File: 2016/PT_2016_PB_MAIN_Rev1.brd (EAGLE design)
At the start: 150.9 x 201.9 mm, 137 parts, among them M1+ ANDERSON_POWERPOLEPP45_PCB_HO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, M1- ANDERSON_POWERPOLEPP45_PCB_HO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, M2+ ANDERSON_POWERPOLEPP45_PCB_HO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, M2- ANDERSON_POWERPOLEPP45_PCB_HO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, M3+ ANDERSON_POWERPOLEPP45_PCB_HO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, M3- ANDERSON_POWERPOLEPP45_PCB_HO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, M4+ ANDERSON_POWERPOLEPP45_PCB_HO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, M4- ANDERSON_POWERPOLEPP45_PCB_HO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, M5+ ANDERSON_POWERPOLEPP45_PCB_HO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, M5- ANDERSON_POWERPOLEPP45_PCB_HO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, M6+ ANDERSON_POWERPOLEPP45_PCB_HO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, M6- ANDERSON_POWERPOLEPP45_PCB_HO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, Q1 Q_IRFS7437PbF, Q11 Q_IRFS7437PbF, Q12 2N7002, Q14 Q_IRFS7437PbF, Q16 Q_IRFS7437PbF, Q2 2N7002, Q20 Q_IRFS7437PbF, Q6 Q_IRFS7437PbF, Q7 Q_IRFS7437PbF, Q9 Q_IRFS7437PbF

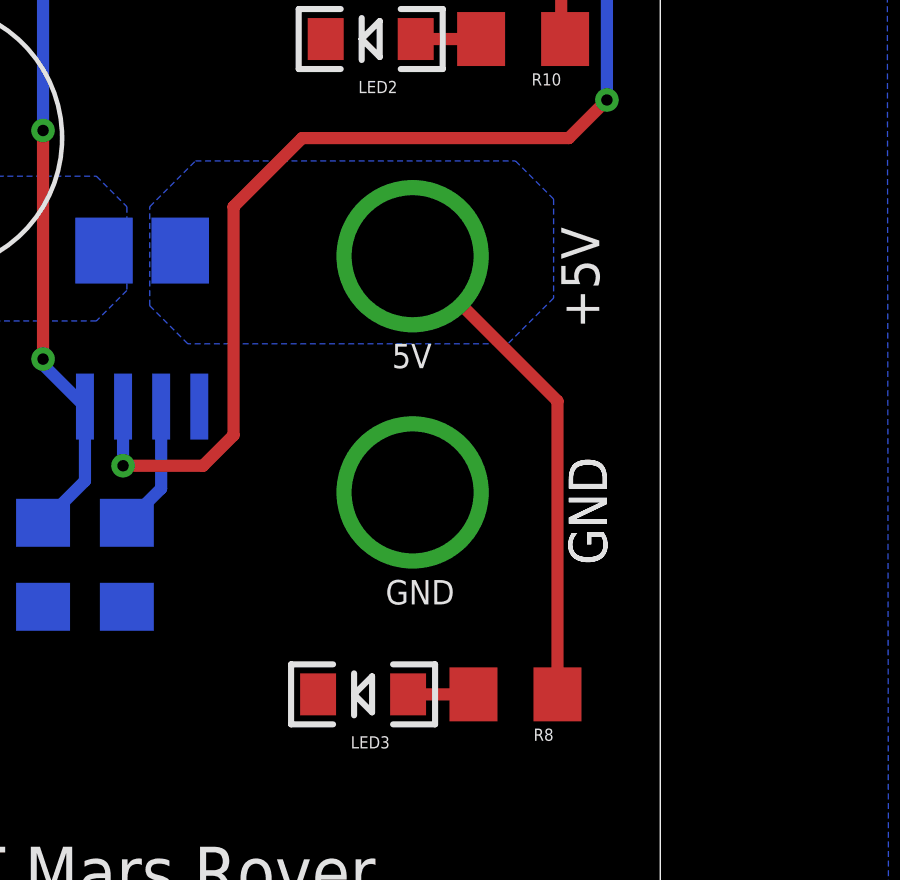
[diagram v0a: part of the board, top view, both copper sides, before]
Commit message: gen gerbers for rev 1
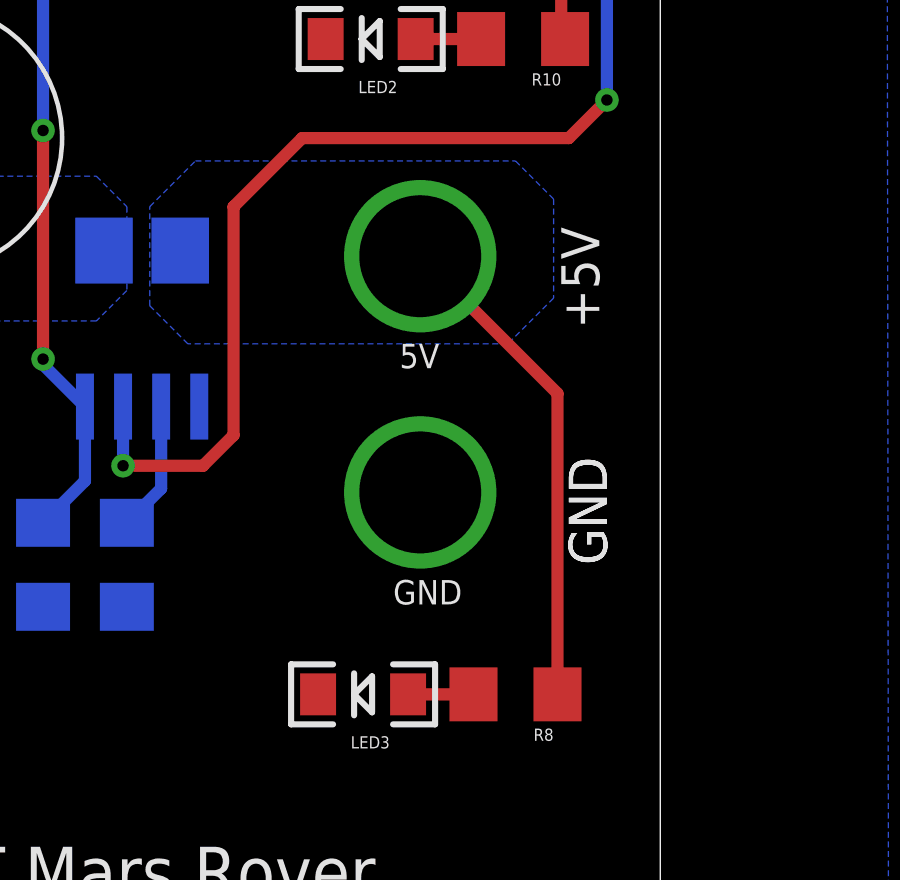
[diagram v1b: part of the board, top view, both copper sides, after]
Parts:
- moved U$45 0.25 mm to (134.1, 14.2)
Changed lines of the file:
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@@
 <layer number="16" name="Bottom" color="1" fill="1" visible="yes" active="yes"/>
 <layer number="17" name="Pads" color="2" fill="1" visible="yes" active="yes"/>
-<layer number="18" name="Vias" color="2" fill="1" visible="no" active="yes"/>
-<layer number="19" name="Unrouted" color="6" fill="1" visible="no" active="yes"/>
-<layer number="20" name="Dimension" color="15" fill="1" visible="no" active="yes"/>
+<layer number="18" name="Vias" color="2" fill="1" visible="yes" active="yes"/>
+<layer number="19" name="Unrouted" color="6" fill="1" visible="yes" active="yes"/>
+<layer number="20" name="Dimension" color="15" fill="1" visible="yes" active="yes"/>
 <layer number="21" name="tPlace" color="7" fill="1" visible="yes" active="yes"/>
-<layer number="22" name="bPlace" color="7" fill="1" visible="no" active="yes"/>
-<layer number="23" name="tOrigins" color="15" fill="1" visible="no" active="yes"/>
-<layer number="24" name="bOrigins" color="15" fill="1" visible="no" active="yes"/>
+<layer number="22" name="bPlace" color="7" fill="1" visible="yes" active="yes"/>
+<layer number="23" name="tOrigins" color="15" fill="1" visible="yes" active="yes"/>
+<layer number="24" name="bOrigins" color="15" fill="1" visible="yes" active="yes"/>
 <layer number="25" name="tNames" color="7" fill="1" visible="no" active="yes"/>
 <layer number="26" name="bNames" color="7" fill="1" visible="no" active="yes"/>
@@
 <layer number="47" name="Measures" color="7" fill="1" visible="no" active="yes"/>
 <layer number="48" name="Document" color="7" fill="1" visible="no" active="yes"/>
-<layer number="49" name="Reference" color="7" fill="1" visible="yes" active="yes"/>
+<layer number="49" name="Reference" color="7" fill="1" visible="no" active="yes"/>
 <layer number="50" name="dxf" color="7" fill="1" visible="no" active="yes"/>
-<layer number="51" name="tDocu" color="7" fill="1" visible="no" active="yes"/>
-<layer number="52" name="bDocu" color="7" fill="1" visible="no" active="yes"/>
+<layer number="51" name="tDocu" color="7" fill="1" visible="yes" active="yes"/>
+<layer number="52" name="bDocu" color="7" fill="1" visible="yes" active="yes"/>
 <layer number="91" name="Nets" color="2" fill="1" visible="no" active="no"/>
 <layer number="92" name="Busses" color="1" fill="1" visible="no" active="no"/>
@@
 <attribute name="COLOR1" value="" x="-16.256" y="4.572" size="1.778" layer="27" display="off"/>
 </element>
-<element name="U$45" library="MRDT-Connectors" package="APP_5V_VERT_CONFIG" value="APP_2POS_CONFIG5V_VERT" x="133.858" y="14.224">
-<attribute name="COLOR2" value="BLACK" x="133.858" y="14.224" size="1.778" layer="27" display="off"/>
-<attribute name="COLOR1" value="RED" x="133.858" y="14.224" size="1.778" layer="27" display="off"/>
+<element name="U$45" library="MRDT-Connectors" package="APP_5V_VERT_CONFIG" value="APP_2POS_CONFIG5V_VERT" x="134.112" y="14.224">
+<attribute name="COLOR2" value="BLACK" x="134.112" y="14.224" size="1.778" layer="27" display="off"/>
+<attribute name="COLOR1" value="RED" x="134.112" y="14.224" size="1.778" layer="27" display="off"/>
 </element>
 <element name="U$46" library="MRDT-Connectors" package="APP_12V_VERT_CONFIG" value="APP_2POS_CONFIG12V_VERT" x="134.112" y="36.068">
@@
 </polygon>
 <contactref element="U$45" pad="VCC"/>
-<wire x1="142.624" y1="12.192" x2="142.624" y2="21.968" width="0.4064" layer="1"/>
-<wire x1="142.624" y1="21.968" x2="137.795" y2="26.797" width="0.4064" layer="1"/>
+<wire x1="142.624" y1="12.192" x2="142.624" y2="22.222" width="0.4064" layer="1"/>
+<wire x1="142.624" y1="22.222" x2="138.049" y2="26.797" width="0.4064" layer="1"/>
 </signal>
 <signal name="N$35">
